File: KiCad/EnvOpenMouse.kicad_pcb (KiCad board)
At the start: 2 copper layers, 34 x 107.5 mm, 74 parts, among them J1 B3U-1000P, J10 0.8mm BM03B, J11 Conn_02x02 Pins, J12 0.8mm BM03B, J13 0.8mm BM03B, J14 0.8mm BM03B, J15 0.8mm BM03B, J16 Conn_01x14, J2 Conn_01x03, J3 B3U-1000P, J4 Conn_02x02 Socket, J5 Conn_02x02 Socket, J6 Conn_02x02 Socket, J7 Conn_02x02 Pins, J8 Conn_02x02 Pins, J9 0.8mm BM03B, SW1 Kailh GM switch, SW2 Kailh GM switch, SW3 Kailh GM switch, SW4 B3U-1000P, SW5 B3U-1000P, SW6 B3U-1000P, SW7 B3U-1000P, SW8 B3U-1000P, SW9 B3U-1000P, U1 AP2112K-3.3, U2 TLV70218DBVR, U3 RP2040, U4 PMW3360DM-T2QU, Y1 3225_4P 12MHz

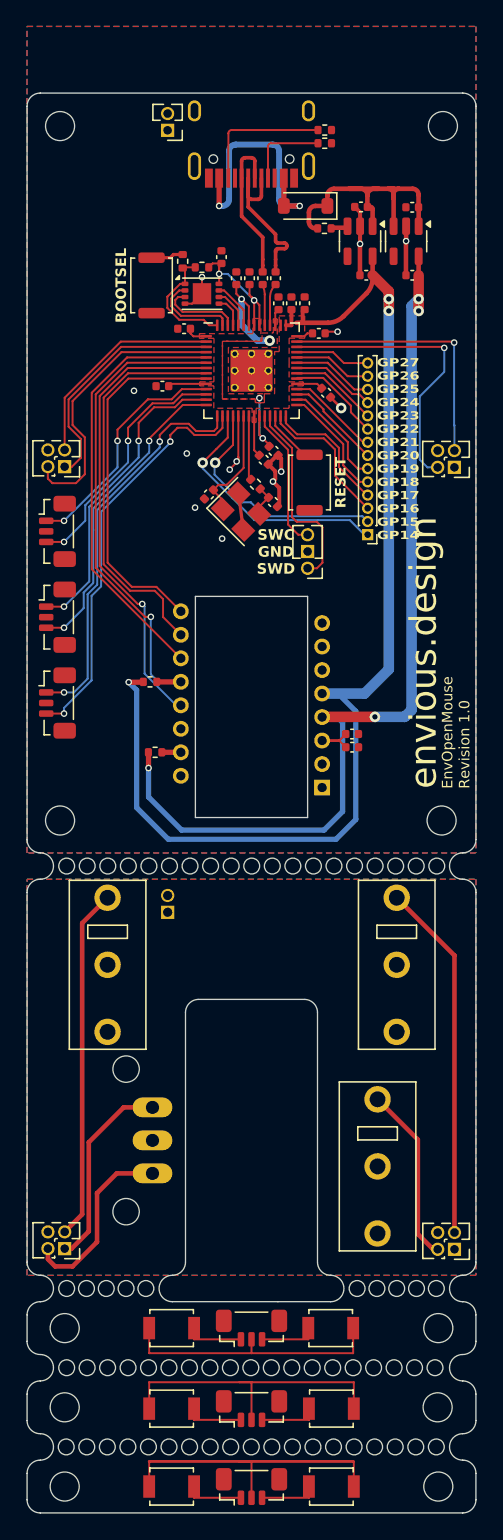
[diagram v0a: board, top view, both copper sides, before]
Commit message: generated fixes production files
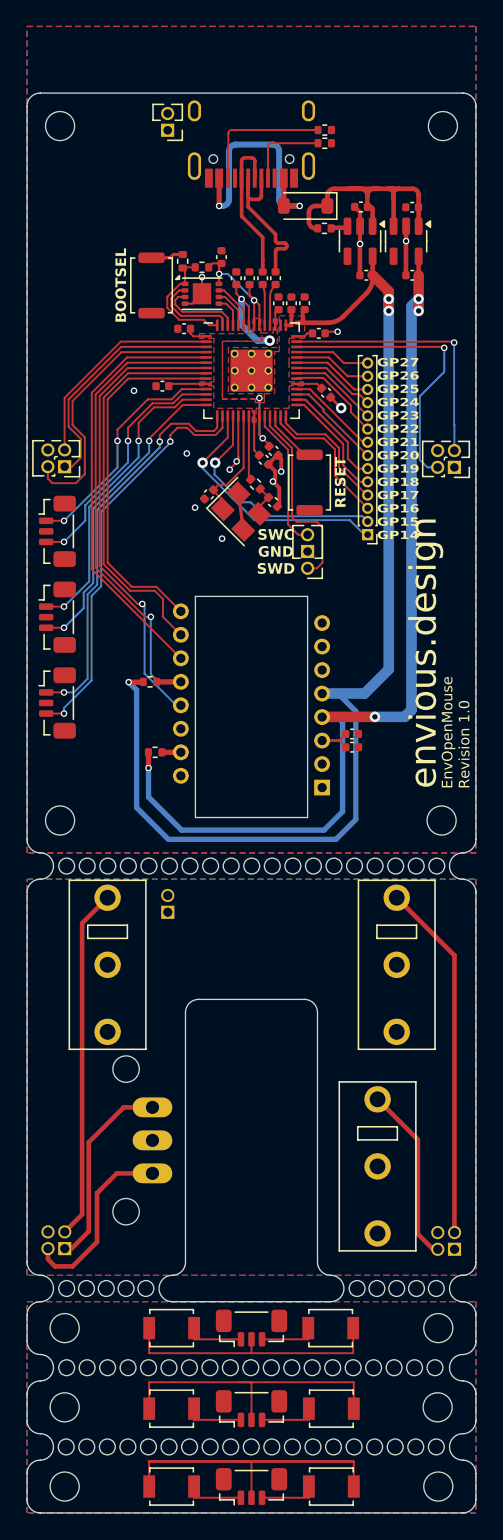
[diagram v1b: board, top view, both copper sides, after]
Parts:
- J5, J6: footprint Connector_PinHeader_1.27mm:PinHeader_2x02_P1.27mm_Vertical -> Connector_PinSocket_1.27mm:PinSocket_2x02_P1.27mm_Vertical; moved to B.Cu
- turned J5 to 0 degrees
- turned J6 to 0 degrees
